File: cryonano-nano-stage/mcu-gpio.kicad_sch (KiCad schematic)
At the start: 18 parts, among them U11 STM32H753ZITx

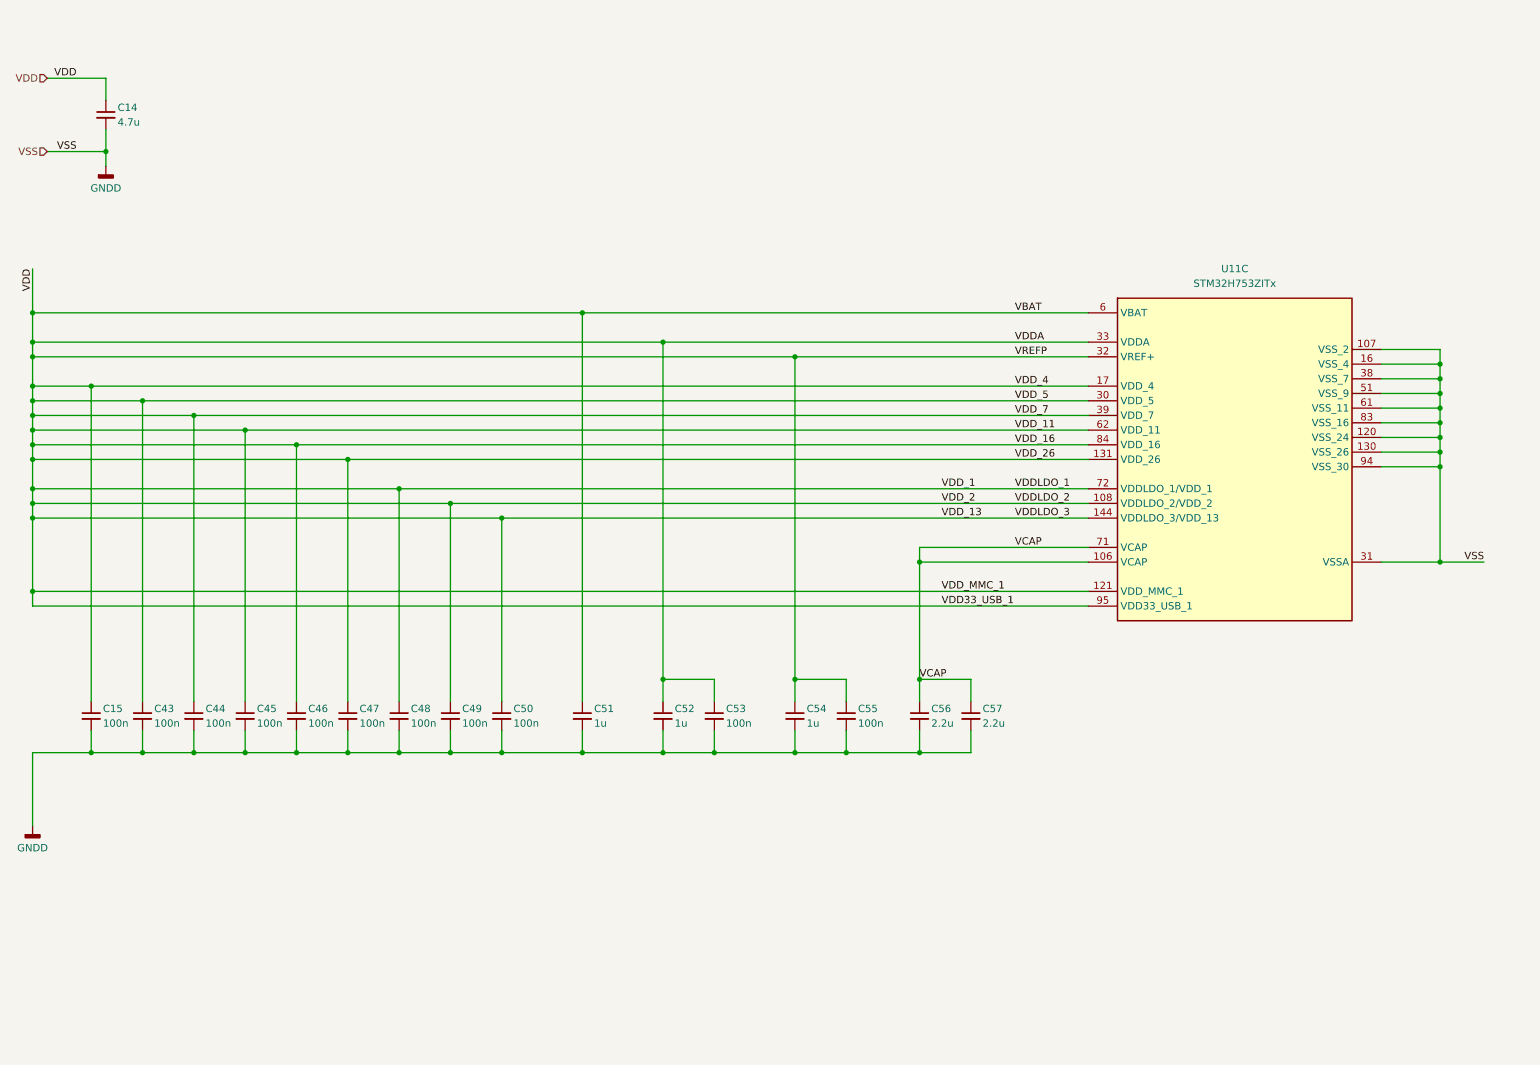
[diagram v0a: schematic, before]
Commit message: sch improved
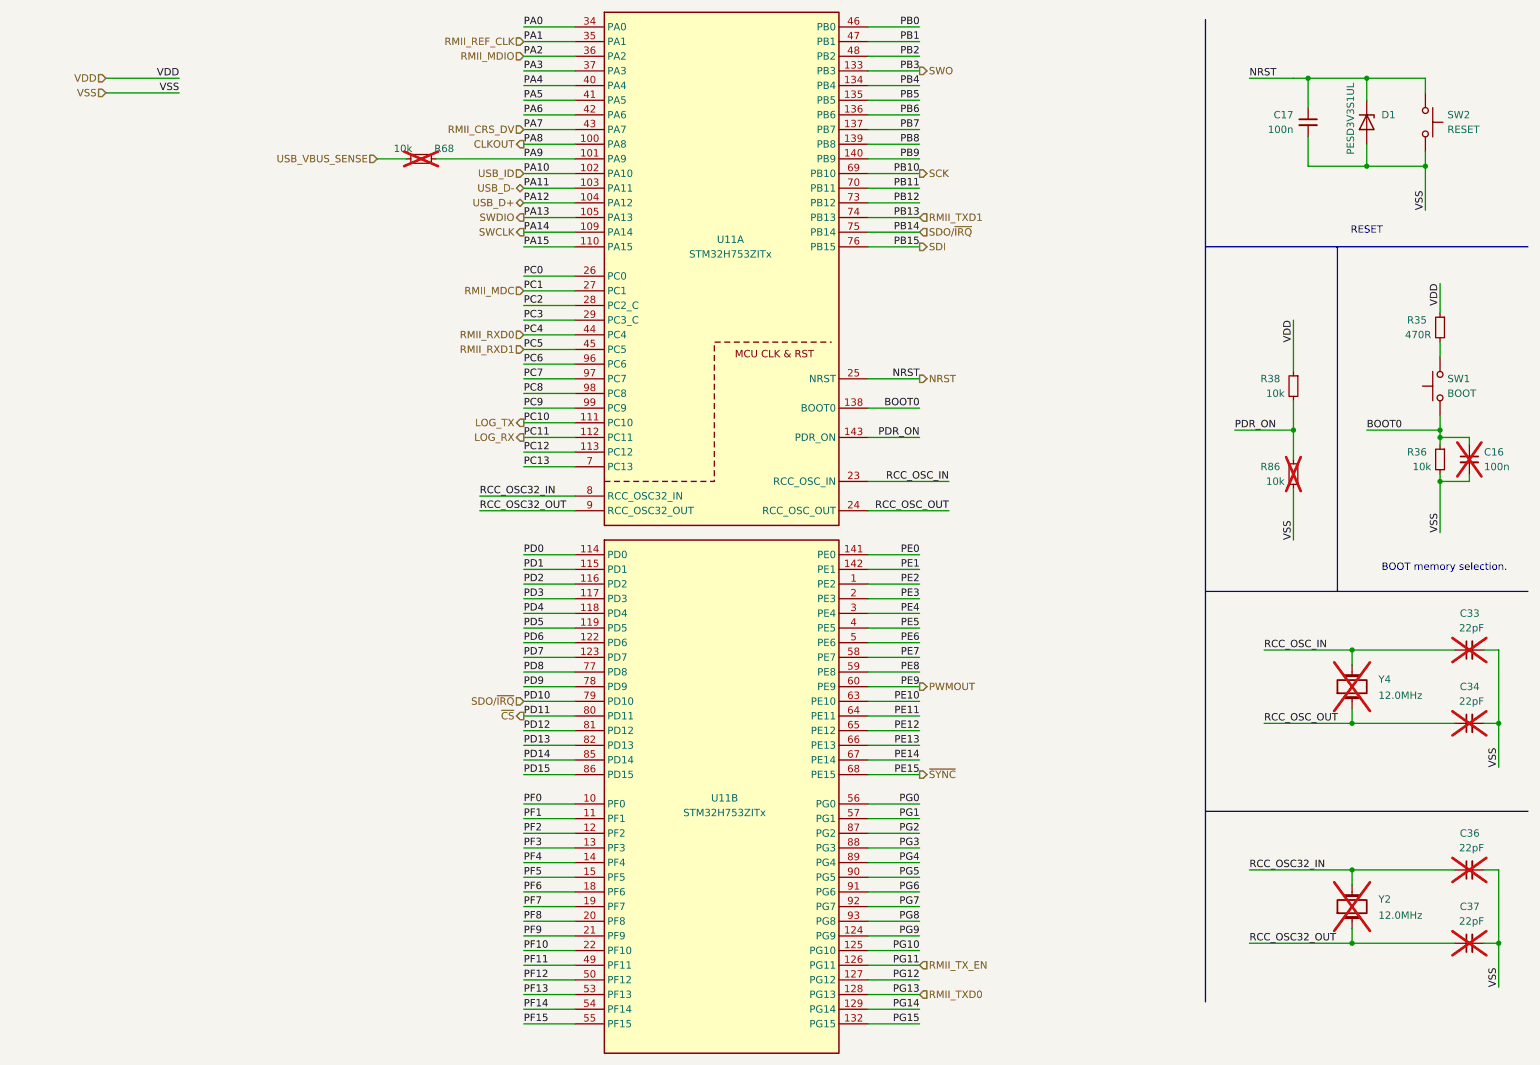
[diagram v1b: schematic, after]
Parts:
- removed C14: 4.7u, Capacitor_SMD:C_0603_1608Metric, symbol Device:C_Small
- removed C15, C43, C44, C45, C46, C47, C48, C49, C50, C53, C55: 100n, Capacitor_SMD:C_0603_1608Metric, symbol Device:C_Small
- removed C51, C52, C54: 1u, Capacitor_SMD:C_0603_1608Metric, symbol Device:C_Small
- removed C56, C57: 2.2u, Capacitor_SMD:C_0603_1608Metric, symbol Device:C_Small
- removed U11: STM32H753ZITx, Package_QFP:LQFP-144_20x20mm_P0.5mm, symbol symbols:STM32H753ZITx
- added C16, C17: 100n, Capacitor_SMD:C_0603_1608Metric, symbol Device:C_Small
- added C33, C34, C36, C37: 22pF, Capacitor_SMD:C_0603_1608Metric, symbol Device:C_Small
- added D1: PESD3V3S1UL, Diode_SMD:D_SOD-882, symbol Diode:PESD3V3S1UL
- added R35: 470R, Resistor_SMD:R_0603_1608Metric, symbol Device:R_Small
- added R36, R38, R68, R86: 10k, Resistor_SMD:R_0603_1608Metric, symbol Device:R_Small
- added SW1: BOOT, Button_Switch_THT:SW_PUSH_6mm, symbol Switch:SW_Push
- added SW2: RESET, Button_Switch_THT:SW_PUSH_6mm, symbol Switch:SW_Push
- added U11: STM32H753ZITx, Package_QFP:LQFP-144_20x20mm_P0.5mm, symbol symbols:STM32H753ZITx
- added Y2, Y4: 12.0MHz, Crystal:Crystal_SMD_3215-2Pin_3.2x1.5mm, symbol Device:Crystal
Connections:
- net VDD: now also R35.1, R38.1
- new net: R35.2, SW1.2
- new net BOOT0: C16.1, R36.1, SW1.1, U11.138 (BOOT0)
- new net CLKOUT: U11.100 (PA8)
- new net LOG_RX: U11.112 (PC11)
- new net LOG_TX: U11.111 (PC10)
- new net NRST: C17.1, D1.1 (K), SW2.1, U11.25 (NRST)
- new net PA0: U11.34 (PA0)
- new net PA15: U11.110 (PA15)
- new net PA3: U11.37 (PA3)
- new net PA4: U11.40 (PA4)
- new net PA5: U11.41 (PA5)
- new net PA6: U11.42 (PA6)
- new net PA9: R68.2, U11.101 (PA9)
- new net PB0: U11.46 (PB0)
- new net PB1: U11.47 (PB1)
- new net PB11: U11.70 (PB11)
- new net PB12: U11.73 (PB12)
- new net PB2: U11.48 (PB2)
- new net PB4: U11.134 (PB4)
- new net PB5: U11.135 (PB5)
- new net PB6: U11.136 (PB6)
- new net PB7: U11.137 (PB7)
- new net PB8: U11.139 (PB8)
- new net PB9: U11.140 (PB9)
- new net PC0: U11.26 (PC0)
- new net PC12: U11.113 (PC12)
- new net PC13: U11.7 (PC13)
- new net PC2: U11.28 (PC2_C)
- new net PC3: U11.29 (PC3_C)
- new net PC6: U11.96 (PC6)
- new net PC7: U11.97 (PC7)
- new net PC8: U11.98 (PC8)
- new net PC9: U11.99 (PC9)
- new net PD0: U11.114 (PD0)
- new net PD1: U11.115 (PD1)
- new net PD12: U11.81 (PD12)
- new net PD13: U11.82 (PD13)
- new net PD14: U11.85 (PD14)
- new net PD15: U11.86 (PD15)
- new net PD2: U11.116 (PD2)
- new net PD3: U11.117 (PD3)
- new net PD4: U11.118 (PD4)
- new net PD5: U11.119 (PD5)
- new net PD6: U11.122 (PD6)
- new net PD7: U11.123 (PD7)
- new net PD8: U11.77 (PD8)
- new net PD9: U11.78 (PD9)
- new net PDR_ON: R38.2, R86.1, U11.143 (PDR_ON)
- new net PE0: U11.141 (PE0)
- new net PE1: U11.142 (PE1)
- new net PE10: U11.63 (PE10)
- new net PE11: U11.64 (PE11)
- new net PE12: U11.65 (PE12)
- new net PE13: U11.66 (PE13)
- new net PE14: U11.67 (PE14)
- new net PE2: U11.1 (PE2)
- new net PE3: U11.2 (PE3)
- new net PE4: U11.3 (PE4)
- new net PE5: U11.4 (PE5)
- new net PE6: U11.5 (PE6)
- new net PE7: U11.58 (PE7)
- new net PE8: U11.59 (PE8)
- new net PF0: U11.10 (PF0)
- new net PF1: U11.11 (PF1)
- new net PF10: U11.22 (PF10)
- new net PF11: U11.49 (PF11)
- new net PF12: U11.50 (PF12)
- new net PF13: U11.53 (PF13)
- new net PF14: U11.54 (PF14)
- new net PF15: U11.55 (PF15)
- new net PF2: U11.12 (PF2)
- new net PF3: U11.13 (PF3)
- new net PF4: U11.14 (PF4)
- new net PF5: U11.15 (PF5)
- new net PF6: U11.18 (PF6)
- new net PF7: U11.19 (PF7)
- new net PF8: U11.20 (PF8)
- new net PF9: U11.21 (PF9)
- new net PG0: U11.56 (PG0)
- new net PG1: U11.57 (PG1)
- new net PG10: U11.125 (PG10)
- new net PG12: U11.127 (PG12)
- new net PG14: U11.129 (PG14)
- new net PG15: U11.132 (PG15)
- new net PG2: U11.87 (PG2)
- new net PG3: U11.88 (PG3)
- new net PG4: U11.89 (PG4)
- new net PG5: U11.90 (PG5)
- new net PG6: U11.91 (PG6)
- new net PG7: U11.92 (PG7)
- new net PG8: U11.93 (PG8)
- new net PG9: U11.124 (PG9)
- new net PWMOUT: U11.60 (PE9)
- new net RCC_OSC32_IN: C36.1, U11.8 (PC14), Y2.2
- new net RCC_OSC32_OUT: C37.1, U11.9 (PC15), Y2.1
- new net RCC_OSC_IN: C33.1, U11.23 (PH0), Y4.2
- new net RCC_OSC_OUT: C34.1, U11.24 (PH1), Y4.1
- new net RMII_CRS_DV: U11.43 (PA7)
- new net RMII_MDC: U11.27 (PC1)
- new net RMII_MDIO: U11.36 (PA2)
- new net RMII_REF_CLK: U11.35 (PA1)
- new net RMII_RXD0: U11.44 (PC4)
- new net RMII_RXD1: U11.45 (PC5)
- new net RMII_TXD0: U11.128 (PG13)
- new net RMII_TXD1: U11.74 (PB13)
- new net RMII_TX_EN: U11.126 (PG11)
- new net SCK: U11.69 (PB10)
- new net SDI: U11.76 (PB15)
- new net SDO/~{IRQ}: U11.75 (PB14), U11.79 (PD10)
- new net SWCLK: U11.109 (PA14)
- new net SWDIO: U11.105 (PA13)
- new net SWO: U11.133 (PB3)
- new net USB_D+: U11.104 (PA12)
- new net USB_D-: U11.103 (PA11)
- new net USB_ID: U11.102 (PA10)
- new net USB_VBUS_SENSE: R68.1
- new net VSS: C16.2, C17.2, C33.2, C34.2, C36.2, C37.2, D1.2 (A), R36.2, R86.2, SW2.2
- new net ~{CS}: U11.80 (PD11)
- new net ~{SYNC}: U11.68 (PE15)
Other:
- note added: "BOOT memory selection."
- note added: "RESET"
